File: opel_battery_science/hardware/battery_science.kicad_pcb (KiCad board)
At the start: 2 copper layers, 68.6 x 62.2 mm, 41 parts, among them P1 CONN_01X08, P6 CONN_01X06, P7 CONN_01X05, P8 CONN_01X05, Q1 BSS84, SW1 SPST, SW2 SPST, U1 BQ76925, U2 LPC11C14, U3 SN74LV4051ADR, U4 MAX11613EUA+

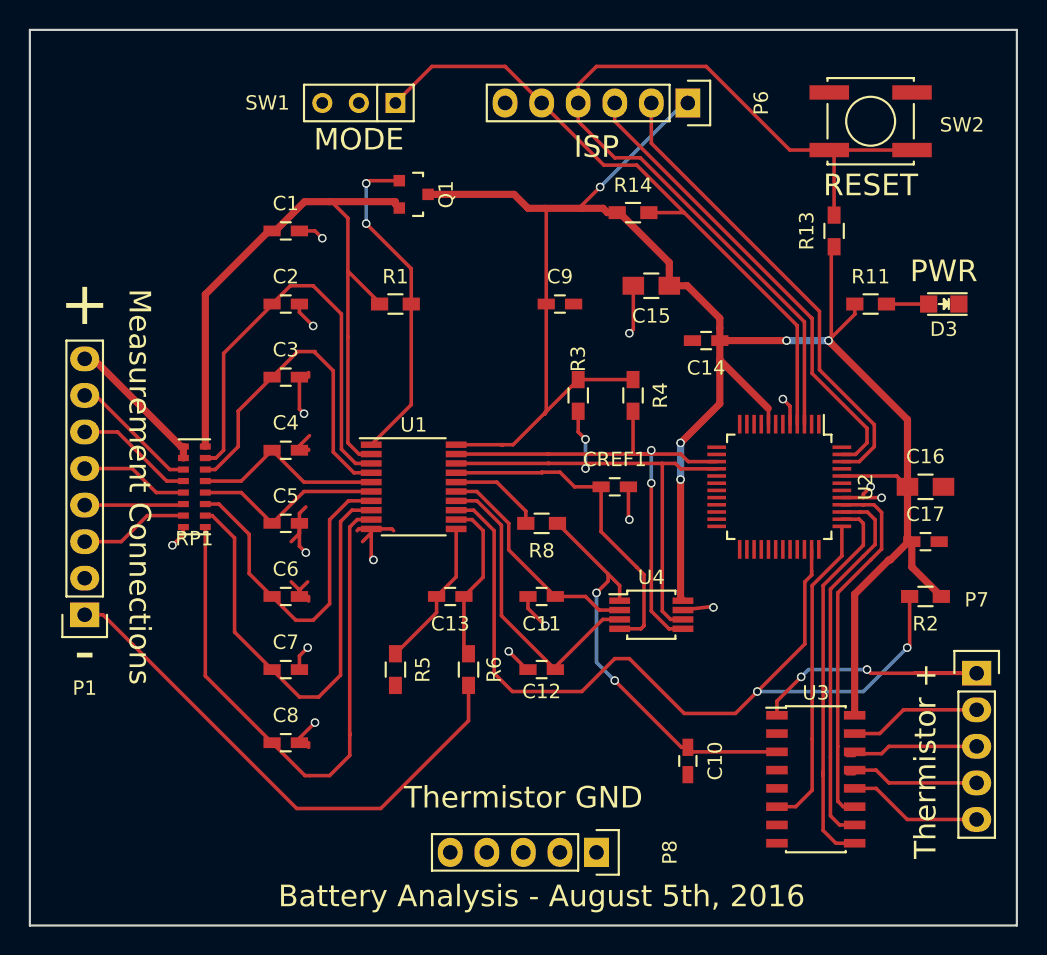
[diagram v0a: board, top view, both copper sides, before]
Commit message: Many fixes, corrected schematic, roughly tried to partition board
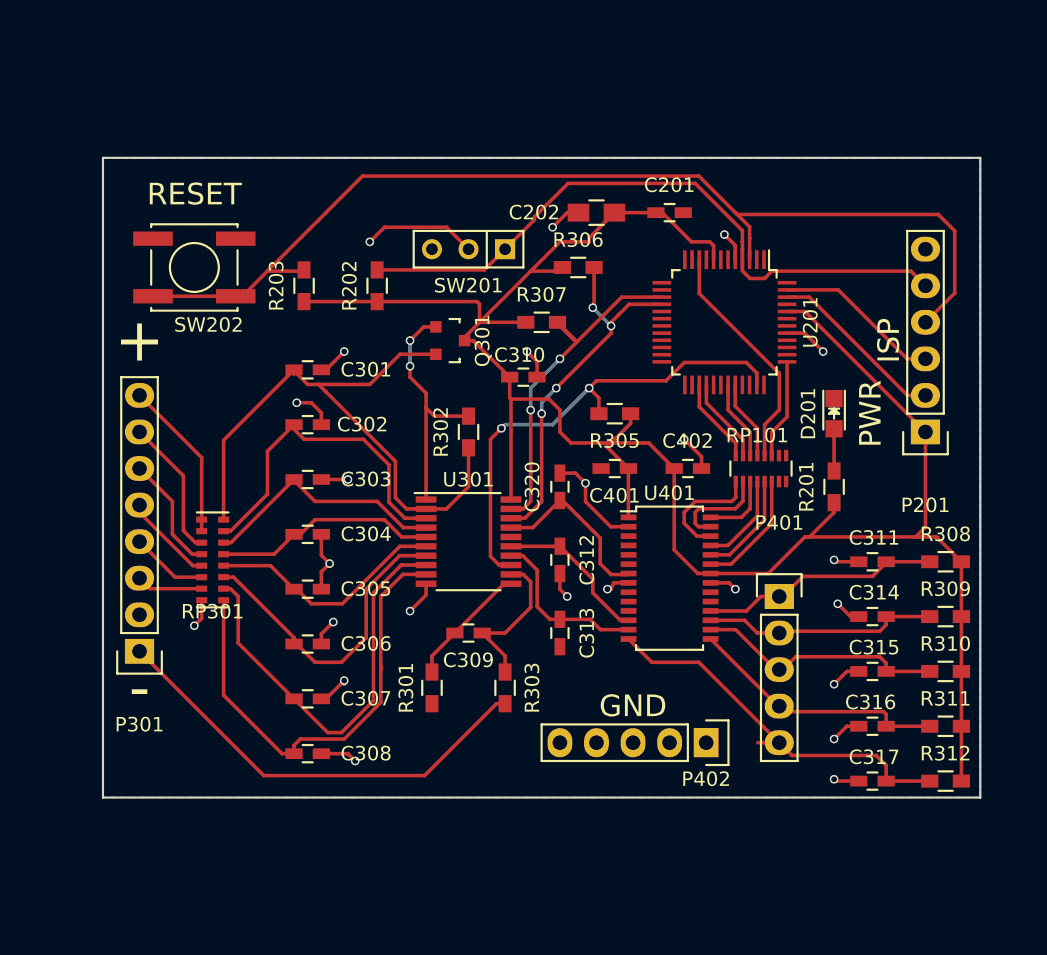
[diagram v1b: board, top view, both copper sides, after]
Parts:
- removed C1: 10μF, Capacitors_SMD:C_0603_HandSoldering
- removed C10: C, Capacitors_SMD:C_0603_HandSoldering
- removed C11, C13, C14, C17: .1μF, Capacitors_SMD:C_0603_HandSoldering
- removed C12: 1nF, Capacitors_SMD:C_0603_HandSoldering
- removed C15, C16: 1μF, Capacitors_SMD:C_0805_HandSoldering
- removed C2, C3, C4, C5, C6, C7, C8, CREF1: 1μF, Capacitors_SMD:C_0603_HandSoldering
- removed C9: 4.7μF, Capacitors_SMD:C_0603_HandSoldering
- removed D3: LED, LEDs:LED_0805
- removed P1: CONN_01X08, Pin_Headers:Pin_Header_Straight_1x08
- removed P6: CONN_01X06, Pin_Headers:Pin_Header_Straight_1x06
- removed P7, P8: CONN_01X05, Pin_Headers:Pin_Header_Straight_1x05
- removed Q1: BSS84, TO_SOT_Packages_SMD:SOT-23
- removed R1: 200k, Resistors_SMD:R_0603_HandSoldering
- removed R11: 100, Resistors_SMD:R_0603_HandSoldering
- removed R13, R14, R8: 10k, Resistors_SMD:R_0603_HandSoldering
- removed R2, R3, R4: 4.7k, Resistors_SMD:R_0603_HandSoldering
- removed R5, R6: 1k, Resistors_SMD:R_0603_HandSoldering
- removed RP1: CAY16-101J8LF, Resistors_SMD:R_Cat16-8
- removed SW1: SPST, Buttons_Switches_ThroughHole:SW_Micro_SPST
- removed SW2: SPST, Buttons_Switches_SMD:SW_SPST_EVPBF
- removed U1: BQ76925, Housings_SSOP:TSSOP-20_4.4x6.5mm_Pitch0.65mm
- removed U2: LPC11C14, Housings_QFP:LQFP-48_7x7mm_Pitch0.5mm
- removed U3: SN74LV4051ADR, Housings_SOIC:SOIC-16_3.9x9.9mm_Pitch1.27mm
- removed U4: MAX11613EUA+, Housings_SSOP:MSOP-8_3x3mm_Pitch0.65mm
- added C201: .1μF, Capacitors_SMD:C_0603_HandSoldering, F.Cu at (161.3, 101.6)
- added C202: 1μF, Capacitors_SMD:C_0805_HandSoldering, F.Cu at (156.2, 101.6)
- added C301: 10μF, Capacitors_SMD:C_0603_HandSoldering, F.Cu at (136.1, 112.5)
- added C302: 1μF, Capacitors_SMD:C_0603_HandSoldering, F.Cu at (136.1, 116.3)
- added C303: 1μF, Capacitors_SMD:C_0603_HandSoldering, F.Cu at (136.1, 120.1)
- added C304: 1μF, Capacitors_SMD:C_0603_HandSoldering, F.Cu at (136.1, 124.0)
- added C305: 1μF, Capacitors_SMD:C_0603_HandSoldering, F.Cu at (136.1, 127.8)
- added C306: 1μF, Capacitors_SMD:C_0603_HandSoldering, F.Cu at (136.1, 131.6)
- added C307: 1μF, Capacitors_SMD:C_0603_HandSoldering, F.Cu at (136.1, 135.4)
- added C308: 1μF, Capacitors_SMD:C_0603_HandSoldering, F.Cu at (136.1, 139.2)
- added C309: .1μF, Capacitors_SMD:C_0603_HandSoldering, F.Cu at (147.3, 130.8)
- added C310: 4.7μF, Capacitors_SMD:C_0603_HandSoldering, F.Cu at (151.1, 113.0)
- added C311: .1μF, Capacitors_SMD:C_0603_HandSoldering, F.Cu at (175.4, 125.9)
- added C312: .1μF, Capacitors_SMD:C_0603_HandSoldering, F.Cu at (153.7, 125.7)
- added C313: 1nF, Capacitors_SMD:C_0603_HandSoldering, F.Cu at (153.7, 130.8)
- added C314: .1μF, Capacitors_SMD:C_0603_HandSoldering, F.Cu at (175.4, 129.7)
- added C315: .1μF, Capacitors_SMD:C_0603_HandSoldering, F.Cu at (175.4, 133.5)
- added C316: .1μF, Capacitors_SMD:C_0603_HandSoldering, F.Cu at (175.4, 137.3)
- added C317: .1μF, Capacitors_SMD:C_0603_HandSoldering, F.Cu at (175.4, 141.1)
- added C320: 1μF, Capacitors_SMD:C_0603_HandSoldering, F.Cu at (153.7, 120.7)
- added C401: 100nF, Capacitors_SMD:C_0603_HandSoldering, F.Cu at (157.5, 119.4)
- added C402: 100nF, Capacitors_SMD:C_0603_HandSoldering, F.Cu at (162.6, 119.4)
- added D201: LED, LEDs:LED_0805, F.Cu at (172.7, 115.6)
- added P201: CONN_01X06, Pin_Headers:Pin_Header_Straight_1x06, F.Cu at (179.1, 116.8)
- added P301: CONN_01X08, Pin_Headers:Pin_Header_Straight_1x08, F.Cu at (124.5, 132.1)
- added P401: CONN_01X05, Pin_Headers:Pin_Header_Straight_1x05, F.Cu at (168.9, 128.3)
- added P402: CONN_01X05, Pin_Headers:Pin_Header_Straight_1x05, F.Cu at (163.8, 138.4)
- added Q301: BSS84, TO_SOT_Packages_SMD:SOT-23, F.Cu at (146.1, 110.5)
- added R201: 100, Resistors_SMD:R_0603_HandSoldering, F.Cu at (172.7, 120.7)
- added R202: 10k, Resistors_SMD:R_0603_HandSoldering, F.Cu at (141.0, 106.7)
- added R203: 10k, Resistors_SMD:R_0603_HandSoldering, F.Cu at (135.9, 106.7)
- added R301: 1k, Resistors_SMD:R_0603_HandSoldering, F.Cu at (144.8, 134.6)
- added R302: 200k, Resistors_SMD:R_0603_HandSoldering, F.Cu at (147.3, 116.8)
- added R303: 1k, Resistors_SMD:R_0603_HandSoldering, F.Cu at (149.9, 134.6)
- added R305: 4.7k, Resistors_SMD:R_0603_HandSoldering, F.Cu at (157.5, 115.6)
- added R306: 4.7k, Resistors_SMD:R_0603_HandSoldering, F.Cu at (154.9, 105.4)
- added R307: 4.7k, Resistors_SMD:R_0603_HandSoldering, F.Cu at (152.4, 109.2)
- added R308: 10k, Resistors_SMD:R_0603_HandSoldering, F.Cu at (180.5, 125.9)
- added R309: 10k, Resistors_SMD:R_0603_HandSoldering, F.Cu at (180.5, 129.7)
- added R310: 10k, Resistors_SMD:R_0603_HandSoldering, F.Cu at (180.5, 133.5)
- added R311: 10k, Resistors_SMD:R_0603_HandSoldering, F.Cu at (180.5, 137.3)
- added R312: 10k, Resistors_SMD:R_0603_HandSoldering, F.Cu at (180.5, 141.1)
- added RP101: 47Ω, Resistors_SMD:R_Array_Convex_8x0602, F.Cu at (167.6, 119.4)
- added RP301: CAY16-101J8LF, Resistors_SMD:R_Cat16-8, F.Cu at (129.5, 125.7)
- added SW201: SPST, Buttons_Switches_ThroughHole:SW_Micro_SPST, F.Cu at (147.3, 104.1)
- added SW202: SPST, Buttons_Switches_SMD:SW_SPST_EVPBF, F.Cu at (128.3, 105.4)
- added U201: LPC11C14, Housings_QFP:LQFP-48_7x7mm_Pitch0.5mm, F.Cu at (165.1, 109.2)
- added U301: BQ76925, Housings_SSOP:TSSOP-20_4.4x6.5mm_Pitch0.65mm, F.Cu at (147.3, 124.5)
- added U401: ADS1148IPWR, Housings_SSOP:TSSOP-28_4.4x9.7mm_Pitch0.65mm, F.Cu at (161.3, 127.0)
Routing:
- net Net-(C1-Pad1): track 49.6 -> 0.00 mm
- net Net-(C301-Pad1): track 0.00 -> 42.9 mm
- net Net-(C8-Pad1): track 41.5 -> 0.00 mm
- net Net-(P1-Pad1): track 37.2 -> 0.00 mm
- net Net-(C308-Pad1): track 0.00 -> 32.6 mm
- net Net-(C7-Pad1): track 32.2 -> 0.00 mm
- net Net-(C2-Pad1): track 31.6 -> 0.00 mm
- net Net-(P301-Pad1): track 0.00 -> 31.0 mm
- net Net-(C307-Pad1): track 0.00 -> 29.3 mm
- net /BatteryMonitoring/COM: track 28.8 -> 0.00 mm, vias 2 -> 0
- net /BatteryMonitoring/ALERT: track 61.8 -> 33.7 mm
- net /ADC/Thermistors/TH5: track 0.00 -> 27.0 mm
- net /Thermistors/C: track 26.9 -> 0.00 mm
- net /Thermistors/B: track 26.4 -> 0.00 mm
- net /Thermistors/A: track 25.7 -> 0.00 mm
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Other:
- board size 68.6 x 62.2 mm -> 61 x 44.5 mm
- board text added: "GND"
- board text removed: "Battery Analysis - August 5th, 2016"
- board text removed: "MODE"
- board text removed: "Measurement Connections"
- board text removed: "Thermistor +"
- board text removed: "Thermistor GND"
